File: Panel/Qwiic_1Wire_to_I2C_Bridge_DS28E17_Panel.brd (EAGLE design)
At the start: 45.7 x 27.9 mm, 23 parts, among them J1 RJ45, J2 RJ45, J3 RJ11, J4 RJ11, U1 DS28E17

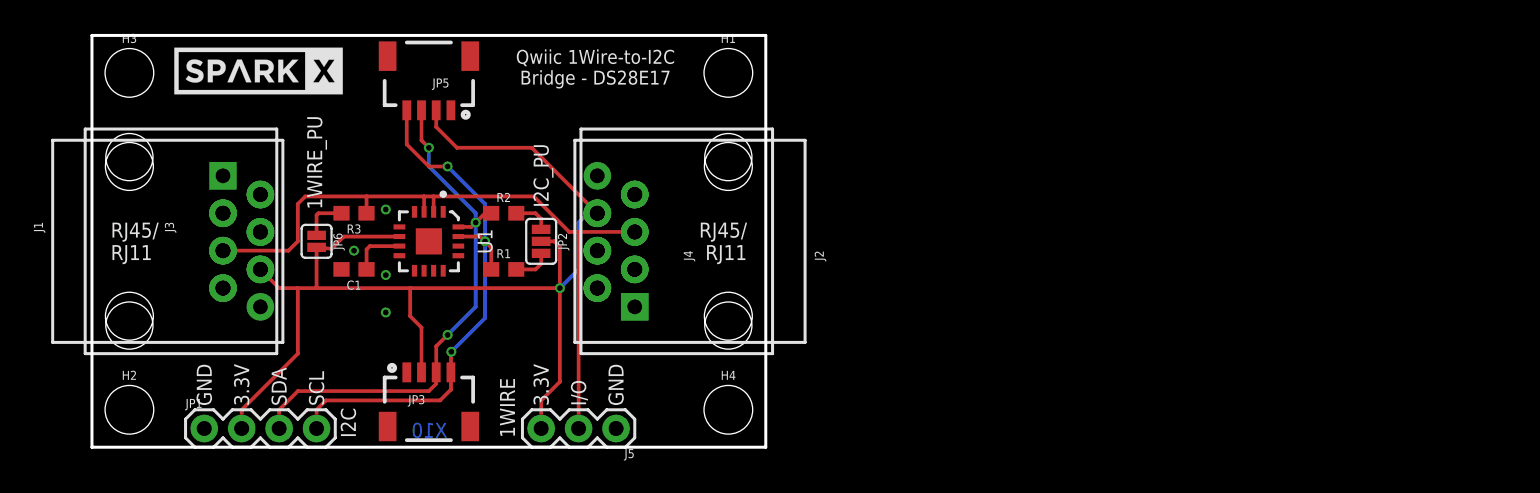
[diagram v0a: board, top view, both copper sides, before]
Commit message: Update to board
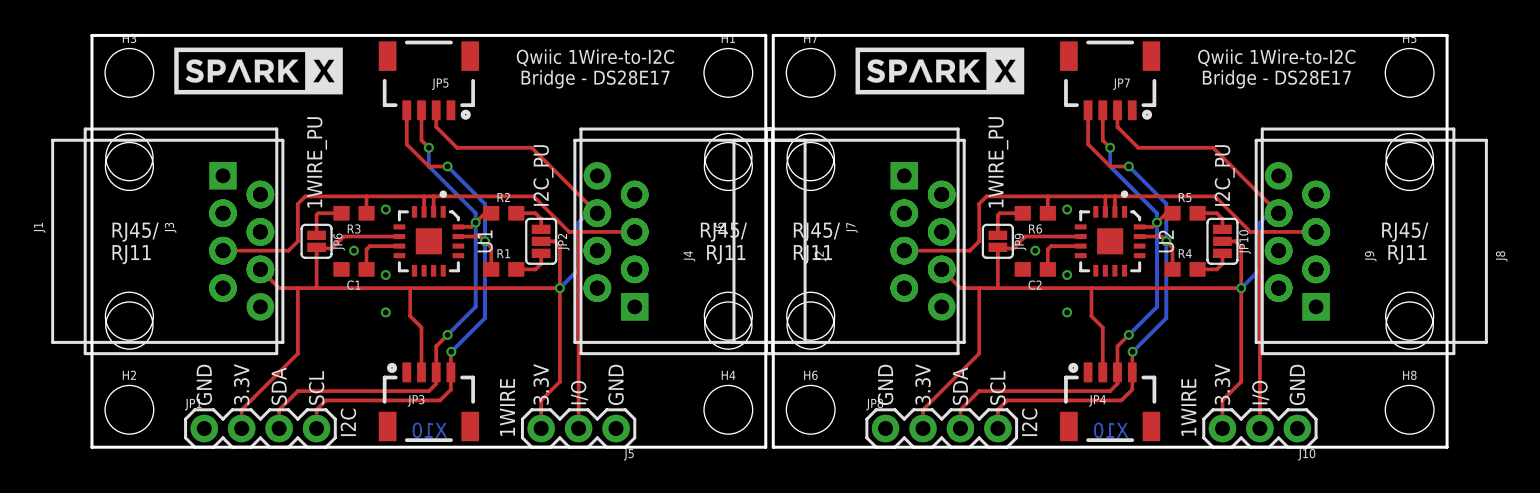
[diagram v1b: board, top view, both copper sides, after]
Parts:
- removed FRAME1: FRAME-LETTER, SparkFun-Aesthetics:CREATIVE_COMMONS
- added C2: 1.0uF, SparkFun-Capacitors:0603
- added H5, H6, H7, H8: STAND-OFF, SparkFun-Hardware:STAND-OFF
- added J10: (no value), SparkFun-Connectors:1X03
- added J6, J8: RJ45, SparkFun-Connectors:RJ45-8
- added J7, J9: RJ11, SparkFun-Connectors:RJ11-6
- added JP10: (no value), SparkFun-Jumpers:SMT-JUMPER_3_2-NC_PASTE_SILK
- added JP4, JP7: (no value), SparkX:1X04_1MM_RA
- added JP8: (no value), SparkX:1X04
- added JP9: (no value), SparkFun-Jumpers:SMT-JUMPER_2_NC_PASTE_SILK
- added LOGO2: OSHW-LOGOM, SparkFun-Aesthetics:OSHW-LOGO-M
- added R4, R5, R6: 4.7k, SparkFun-Resistors:0603
- added U$1, U$4: SPARKX-LOGO5, SparkX:SPARKX-LARGE
- added U2: DS28E17, SparkX:TQFN-16
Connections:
- new net 3.3V1: J10.3, J6.6, J7.5, J8.6, J9.5, JP10.2, JP4.2, JP7.2, JP8.2, JP9.2, U2.6
- new net AWAKE1: U2.12
- new net BUSY1: U2.13
- new net ED1: U2.5
- new net GND1: C2.2, J10.1, J6.4, J7.3, J8.4, J9.3, JP4.1, JP7.1, JP8.1, U2.4, U2.8
- new net IO1: J10.2, J6.5, J7.4, J8.5, J9.4, R6.1, U2.2, U2.3
- new net N$5: C2.1, U2.7
- new net N$6: JP9.1, R6.2
- new net N$7: JP10.1, R5.2
- new net N$8: JP10.3, R4.2
- new net SCL1: JP4.4, JP7.4, JP8.4, R4.1, U2.15
- new net SDA1: JP4.3, JP7.3, JP8.3, R5.1, U2.16
- new net XD1: U2.14
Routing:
- net 3.3V1: track 0.00 -> 82.0 mm, vias 0 -> 1
- net IO1: track 0.00 -> 48.5 mm
- net SCL1: track 0.00 -> 37.8 mm, vias 0 -> 3
- net SDA1: track 0.00 -> 36.5 mm, vias 0 -> 3
- net N$5: track 0.00 -> 3.68 mm
- net N$6: track 0.00 -> 3.11 mm
- net N$8: track 0.00 -> 2.56 mm
- net N$7: track 0.00 -> 2.56 mm
- added copper zone on layer 1, net GND1
- added copper zone on layer 16, net GND1
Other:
- board size 45.7 x 27.9 mm -> 91.9 x 27.9 mm
- board text removed: "Joel Bartlett"
